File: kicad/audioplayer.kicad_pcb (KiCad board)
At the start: 2 copper layers, 100 x 75 mm, 43 parts, among them J1 Panel, J2 Charge_USB, J3 Speakers, J4 RFID, SW1 POWER, U1 PB-500, U2 ESP32-nodeMCU, U3 OLED, U4 GY-521, U5 VS1053/SD_breakout, U6 ULN2003, U7 HW-323

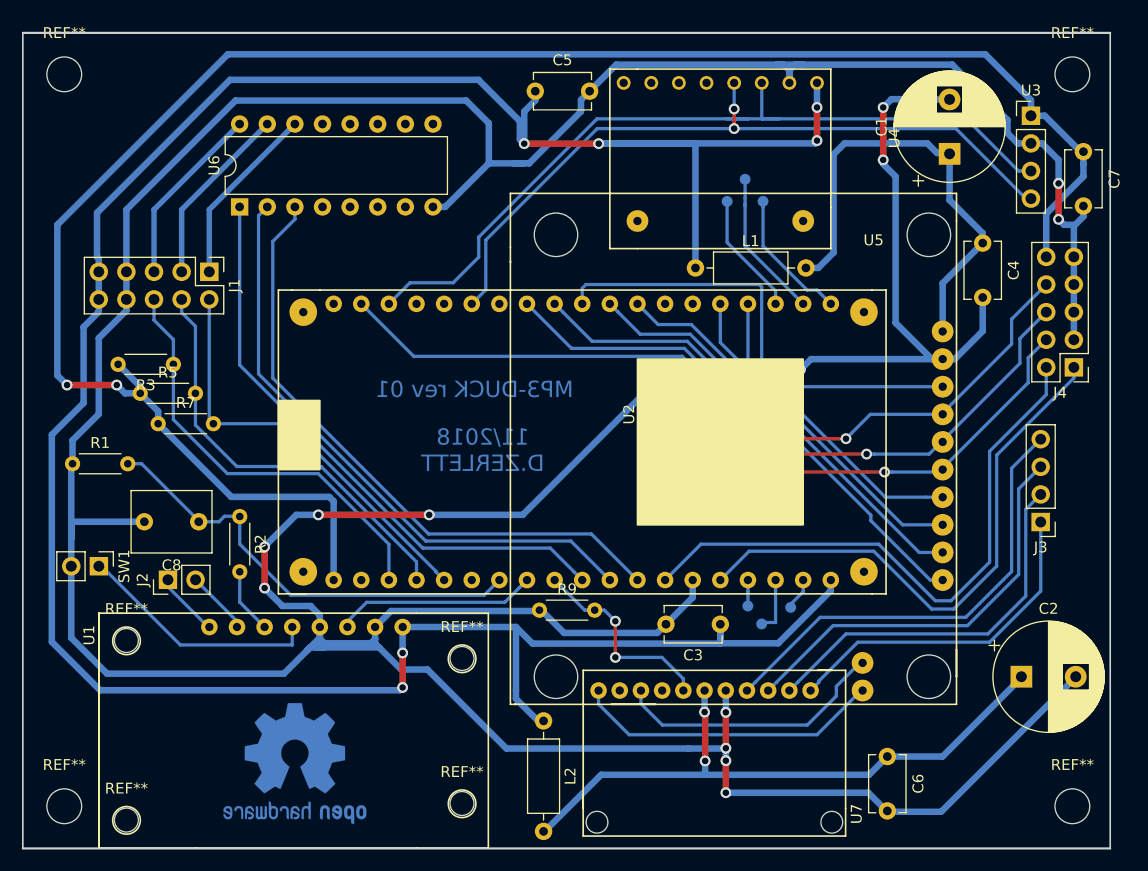
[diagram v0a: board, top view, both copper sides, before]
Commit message: board rev 02
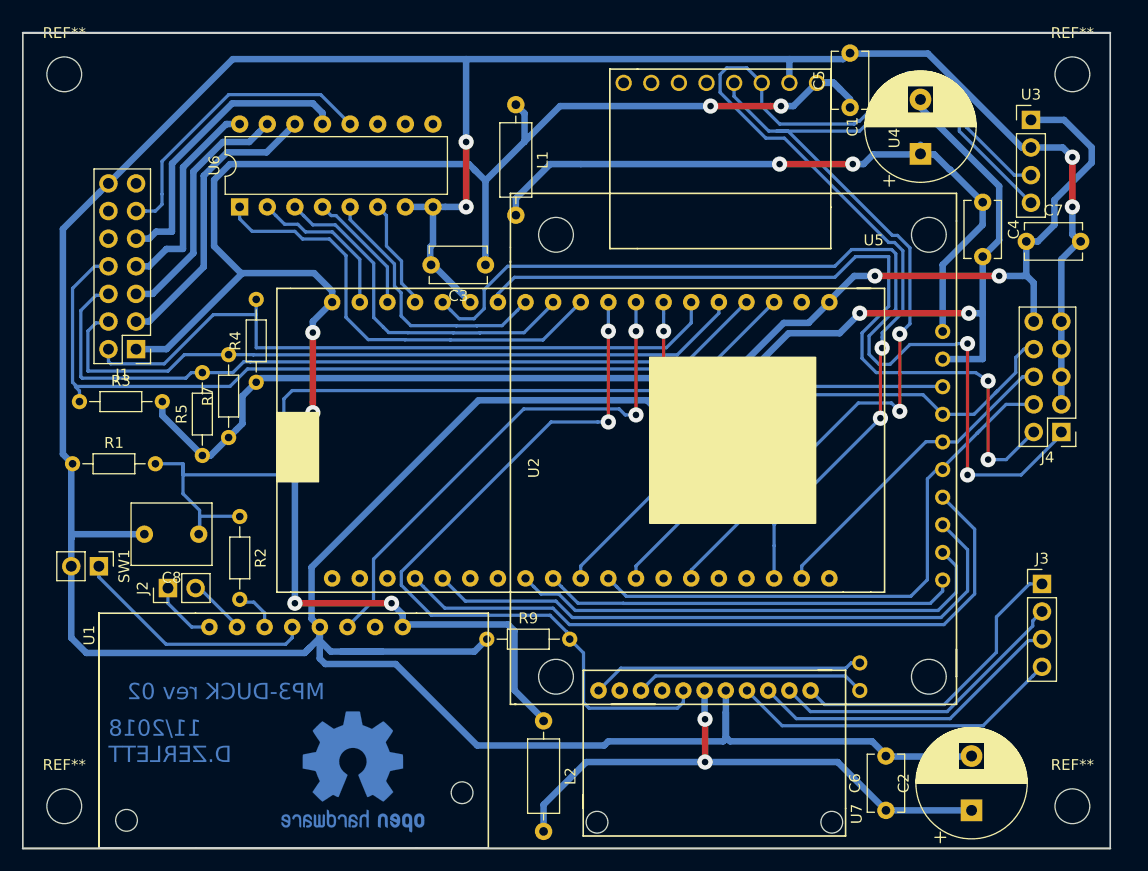
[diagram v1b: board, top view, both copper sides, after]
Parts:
- removed the REF** at (92.8, 92.7)
- removed the REF** at (31.7, 95.7)
- removed the REF** at (87.0, 55.3)
- removed the REF** at (90.2, 94.2)
- removed the REF** at (88.9, 92.6)
- removed the REF** at (88.6, 53.3)
- removed the REF** at (90.3, 55.3)
- removed the REF** at (31.7, 112.2)
- removed the REF** at (62.6, 110.7)
- removed the REF** at (62.6, 97.4)
- added R4: 4.7k, Resistor_THT:R_Axial_DIN0204_L3.6mm_D1.6mm_P7.62mm_Horizontal, F.Cu at (43.7, 72.0)
- J1: footprint Connector_PinHeader_2.54mm:PinHeader_2x05_P2.54mm_Vertical -> Connector_PinHeader_2.54mm:PinHeader_2x07_P2.54mm_Vertical
- R1, R2, R3, R5, R7, R9: footprint Resistor_THT:R_Axial_DIN0204_L3.6mm_D1.6mm_P5.08mm_Horizontal -> Resistor_THT:R_Axial_DIN0204_L3.6mm_D1.6mm_P7.62mm_Horizontal
- U2: footprint audioplayer:esp32-nodemcu -> audioplayer:esp32-nodemcu-noholes
- U4: footprint audioplayer:gy-521 -> audioplayer:gy-521-noholes
- moved C3 39.5 mm to (64.8, 61.2)
- moved C5 29.0 mm to (98.3, 46.7), turned to 90 degrees
- moved L1 22.3 mm to (67.6, 46.5), turned to 270 degrees
- moved C2 13.1 mm to (109.5, 111.4), turned to 90 degrees
- moved J1 9.79 mm to (32.6, 68.9), turned to 180 degrees
- moved C7 9.79 mm to (114.5, 59.0), turned to 0 degrees
- moved R3 9.29 mm to (27.4, 73.8), turned to 0 degrees
- moved U2 9.19 mm to (69.7, 79.9), turned to 270 degrees
- moved R5 8.08 mm to (38.7, 78.7), turned to 90 degrees
- moved R7 6.60 mm to (41.1, 77.1), turned to 90 degrees
- moved J4 6.05 mm to (117.7, 76.6)
- moved J3 5.69 mm to (115.9, 90.5), turned to 0 degrees
- moved R9 5.52 mm to (64.9, 95.6)
- moved REF** 5.39 mm to (52.6, 107.8)
- moved C6 4.95 mm to (101.6, 111.4), turned to 90 degrees
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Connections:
- J1 pad 1: /LED3_OD -> +5V
- J1 pad 10: +5V -> Net-(J1-Pad10)
- J1 pad 2: SW3 -> SW4
- J1 pad 3: /LED2_OD -> /LED4_OD
- J1 pad 4: SW2 -> SW3
- J1 pad 5: /LED1_OD -> /LED3_OD
- J1 pad 6: SW1 -> SW2
- J1 pad 7: GND -> /LED2_OD
- J1 pad 8: GND -> SW1
- J1 pad 9: +5V -> /LED1_OD
- U1 pad 7: GND -> Net-(U1-Pad7)
- U2 pad 16: Net-(U2-Pad16) -> LED4
- U2 pad 17: Net-(U2-Pad17) -> LED5
- U2 pad 18: Net-(U2-Pad18) -> LED6
- U2 pad 6: Net-(U2-Pad6) -> SW4
- U6 pad 12: Net-(U6-Pad12) -> Net-(J1-Pad11)
- U6 pad 13: Net-(U6-Pad13) -> /LED1_OD
- U6 pad 14: /LED3_OD -> /LED4_OD
- U6 pad 15: /LED2_OD -> /LED3_OD
- U6 pad 16: /LED1_OD -> /LED2_OD
- U6 pad 2: LED2 -> LED6
- U6 pad 3: LED3 -> LED2
- U6 pad 4: Net-(U6-Pad4) -> LED5
- U6 pad 5: Net-(U6-Pad5) -> LED3
- U6 pad 6: Net-(U6-Pad6) -> LED4
- U6 pad 7: Net-(U6-Pad7) -> GND
- U7 pad 11: Net-(U5-Pad12) -> Net-(U5-Pad11)
- U7 pad 9: Net-(U5-Pad11) -> Net-(U5-Pad12)
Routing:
- net +5V: track 242.6 -> 172.3 mm
- net SW4: track 0.00 -> 64.0 mm
- net +3V3: track 172.2 -> 117.3 mm
- net /AMP_ENABLE: track 19.0 -> 71.8 mm
- net /MOSI: track 76.3 -> 29.7 mm, vias 2 -> 0
- net SW1: track 39.7 -> 82.3 mm
- net /RST: track 51.6 -> 89.1 mm, vias 0 -> 2
- net /MP3_XCS: track 28.2 -> 64.5 mm
- net /ADC_BATT: track 41.7 -> 76.7 mm, vias 0 -> 2
- net SW2: track 39.3 -> 73.4 mm
- net GND: track 468.3 -> 434.3 mm, vias 14 -> 6
- net LED3: track 57.8 -> 24.7 mm
- net /LOW_BATT: track 18.1 -> 47.7 mm, vias 0 -> 2
- net SW3: track 38.8 -> 67.1 mm
- net /SDA: track 67.9 -> 96.1 mm
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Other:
- net class 5V: via_dia 1 -> 1.4
- net class Default: via_dia 1 -> 1.4
- net class GND removed
- net class VCC_AMP removed
- net class thicker removed
- rule via_min_size: 0.8 -> 1.4
- board text added: "MP3-DUCK rev 02"
- board text removed: "MP3-DUCK rev 01"
